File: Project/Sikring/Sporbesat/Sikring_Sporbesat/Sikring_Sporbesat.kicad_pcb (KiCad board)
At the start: 2 copper layers, 79 x 80 mm, 72 parts, among them J1 Screw_Terminal_01x02, J2 Screw_Terminal_01x08, Q1 BC857, Q2 BC847, Q3 BC857, Q4 BC847, Q5 BC857, Q6 BC847, Q7 BC857, Q8 BC847, U1 PC847

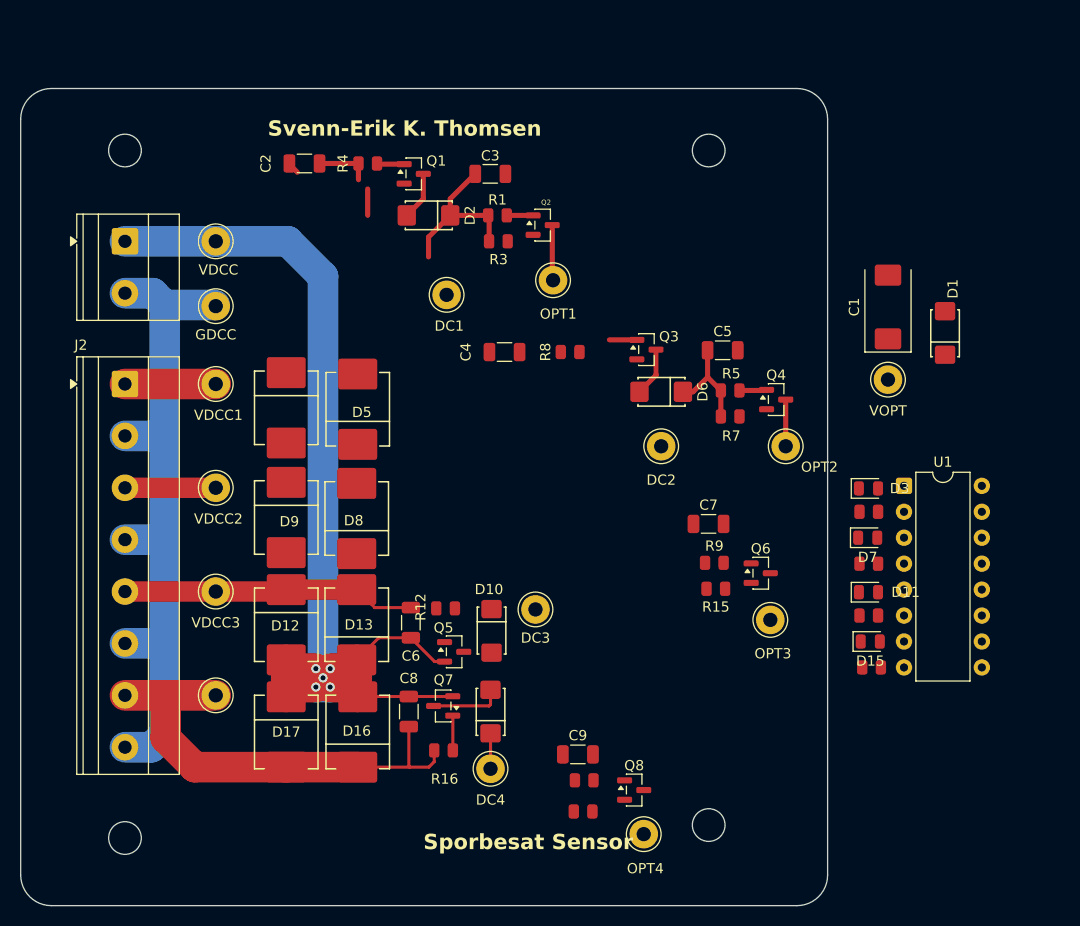
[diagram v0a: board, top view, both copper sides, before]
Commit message: NYT PCB
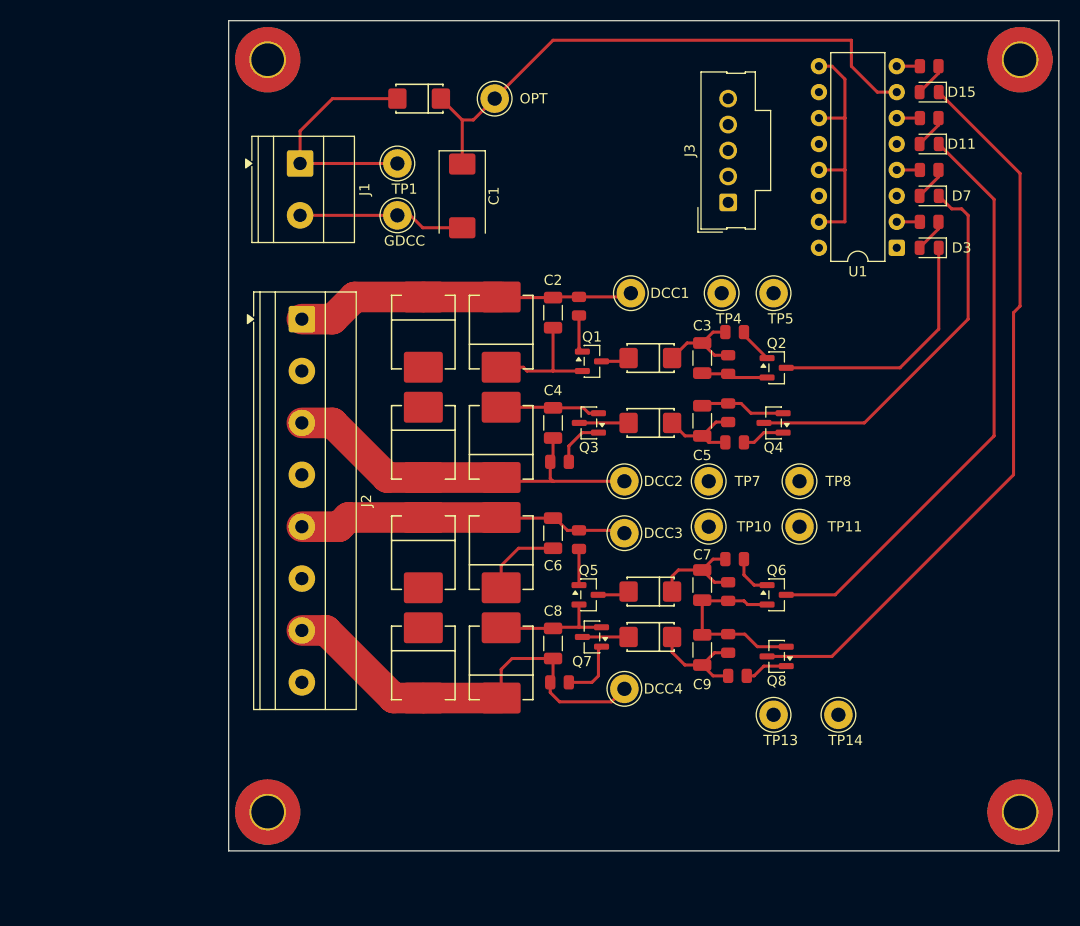
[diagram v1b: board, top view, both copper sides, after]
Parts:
- removed REF** (x4): MountingHole_3.2mm_M3, MountingHole:MountingHole_3.2mm_M3
- removed TP12: VDCC3, TestPoint:TestPoint_Loop_D2.60mm_Drill1.4mm_Beaded
- removed TP15: VDCC4, TestPoint:TestPoint_Loop_D2.60mm_Drill1.4mm_Beaded
- removed TP2: VOPT, TestPoint:TestPoint_Loop_D2.60mm_Drill1.4mm_Beaded
- removed TP3: GDCC, TestPoint:TestPoint_Loop_D2.60mm_Drill1.4mm_Beaded
- removed TP6: VDCC1, TestPoint:TestPoint_Loop_D2.60mm_Drill1.4mm_Beaded
- removed TP9: VDCC2, TestPoint:TestPoint_Loop_D2.60mm_Drill1.4mm_Beaded
- added DCC1: VDCC1, TestPoint:TestPoint_Loop_D2.60mm_Drill1.4mm_Beaded, F.Cu at (78.7, 66.0)
- added DCC2: VDCC2, TestPoint:TestPoint_Loop_D2.60mm_Drill1.4mm_Beaded, F.Cu at (78.1, 84.5)
- added DCC3: VDCC3, TestPoint:TestPoint_Loop_D2.60mm_Drill1.4mm_Beaded, F.Cu at (78.1, 89.5)
- added DCC4: VDCC4, TestPoint:TestPoint_Loop_D2.60mm_Drill1.4mm_Beaded, F.Cu at (78.1, 104.8)
- added GDCC: GDCC, TestPoint:TestPoint_Loop_D2.60mm_Drill1.4mm_Beaded, F.Cu at (55.9, 58.4)
- added H1: MountingHole_Pad, MountingHole:MountingHole_3.2mm_M3_Pad_TopBottom, F.Cu at (43.2, 43.2)
- added H2: MountingHole_Pad, MountingHole:MountingHole_3.2mm_M3_Pad_TopBottom, F.Cu at (116.8, 43.2)
- added H3: MountingHole_Pad, MountingHole:MountingHole_3.2mm_M3_Pad_TopBottom, F.Cu at (43.2, 116.8)
- added H4: MountingHole_Pad, MountingHole:MountingHole_3.2mm_M3_Pad_TopBottom, F.Cu at (116.8, 116.8)
- added J3: Conn_01x05_Pin, Connector_Molex:Molex_SL_171971-0005_1x05_P2.54mm_Vertical, F.Cu at (88.3, 57.1)
- added OPT: VOPT, TestPoint:TestPoint_Loop_D2.60mm_Drill1.4mm_Beaded, F.Cu at (65.4, 47.0)
- moved R14 59.1 mm to (107.9, 43.8), turned to 0 degrees
- moved D1 56.4 mm to (58.0, 47.0), turned to 180 degrees
- moved D15 54.1 mm to (107.9, 46.4), turned to 180 degrees
- moved R10 49.1 mm to (107.9, 48.9), turned to 0 degrees
- moved D11 44.3 mm to (107.9, 51.4), turned to 180 degrees
- moved C1 43.1 mm to (62.2, 56.5), turned to -90 degrees
- moved R6 39.0 mm to (107.9, 54.0), turned to 0 degrees
- moved D7 34.0 mm to (107.9, 56.5), turned to 180 degrees
- moved R2 29.0 mm to (107.9, 59.1)
- moved C2 28.4 mm to (71.1, 67.9), turned to 90 degrees
- moved TP13 28.2 mm to (92.7, 107.3)
- moved C3 27.5 mm to (85.7, 72.4), turned to -90 degrees
- moved TP4 26.9 mm to (87.6, 66.0)
- moved Q2 26.8 mm to (93.0, 73.3)
- moved R1 25.9 mm to (88.9, 69.8)
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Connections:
- U1 pad 10: BESAT4 -> Net-(J3-Pin_4)
- U1 pad 12: BESAT3 -> Net-(J3-Pin_3)
- U1 pad 14: BESAT2 -> Net-(J3-Pin_2)
- U1 pad 16: BESAT1 -> Net-(J3-Pin_1)
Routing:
- net Net-(D15-K): track 0.00 -> 72.5 mm
- net Net-(D11-K): track 0.00 -> 57.6 mm
- net VOPT: track 0.00 -> 56.6 mm
- net VDCC: track 107.4 -> 66.0 mm, vias 5 -> 0
- net Net-(D7-K): track 4.57 -> 38.0 mm
- net VDCC2: track 8.89 -> 38.4 mm
- net GDIGI: track 0.00 -> 24.7 mm
- net Net-(D3-K): track 5.43 -> 24.5 mm
- net GDCC: track 68.0 -> 50.0 mm
- net VDCC1: track 16.9 -> 33.3 mm
- net Net-(D10-K): track 0.00 -> 10.4 mm
- net Net-(D14-K): track 3.47 -> 11.0 mm
- net Net-(D2-K): track 16.3 -> 9.30 mm
- net Net-(Q8-B): track 0.00 -> 4.26 mm
- net Net-(Q6-B): track 0.00 -> 4.22 mm
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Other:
- board size 79 x 80 mm -> 81.3 x 81.3 mm
- board text removed: "Sporbesat Sensor"
- board text removed: "Svenn-Erik K. Thomsen"
